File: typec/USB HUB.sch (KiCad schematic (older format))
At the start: 36 parts, among them U7 USB_HUB, Y1 24 MHz

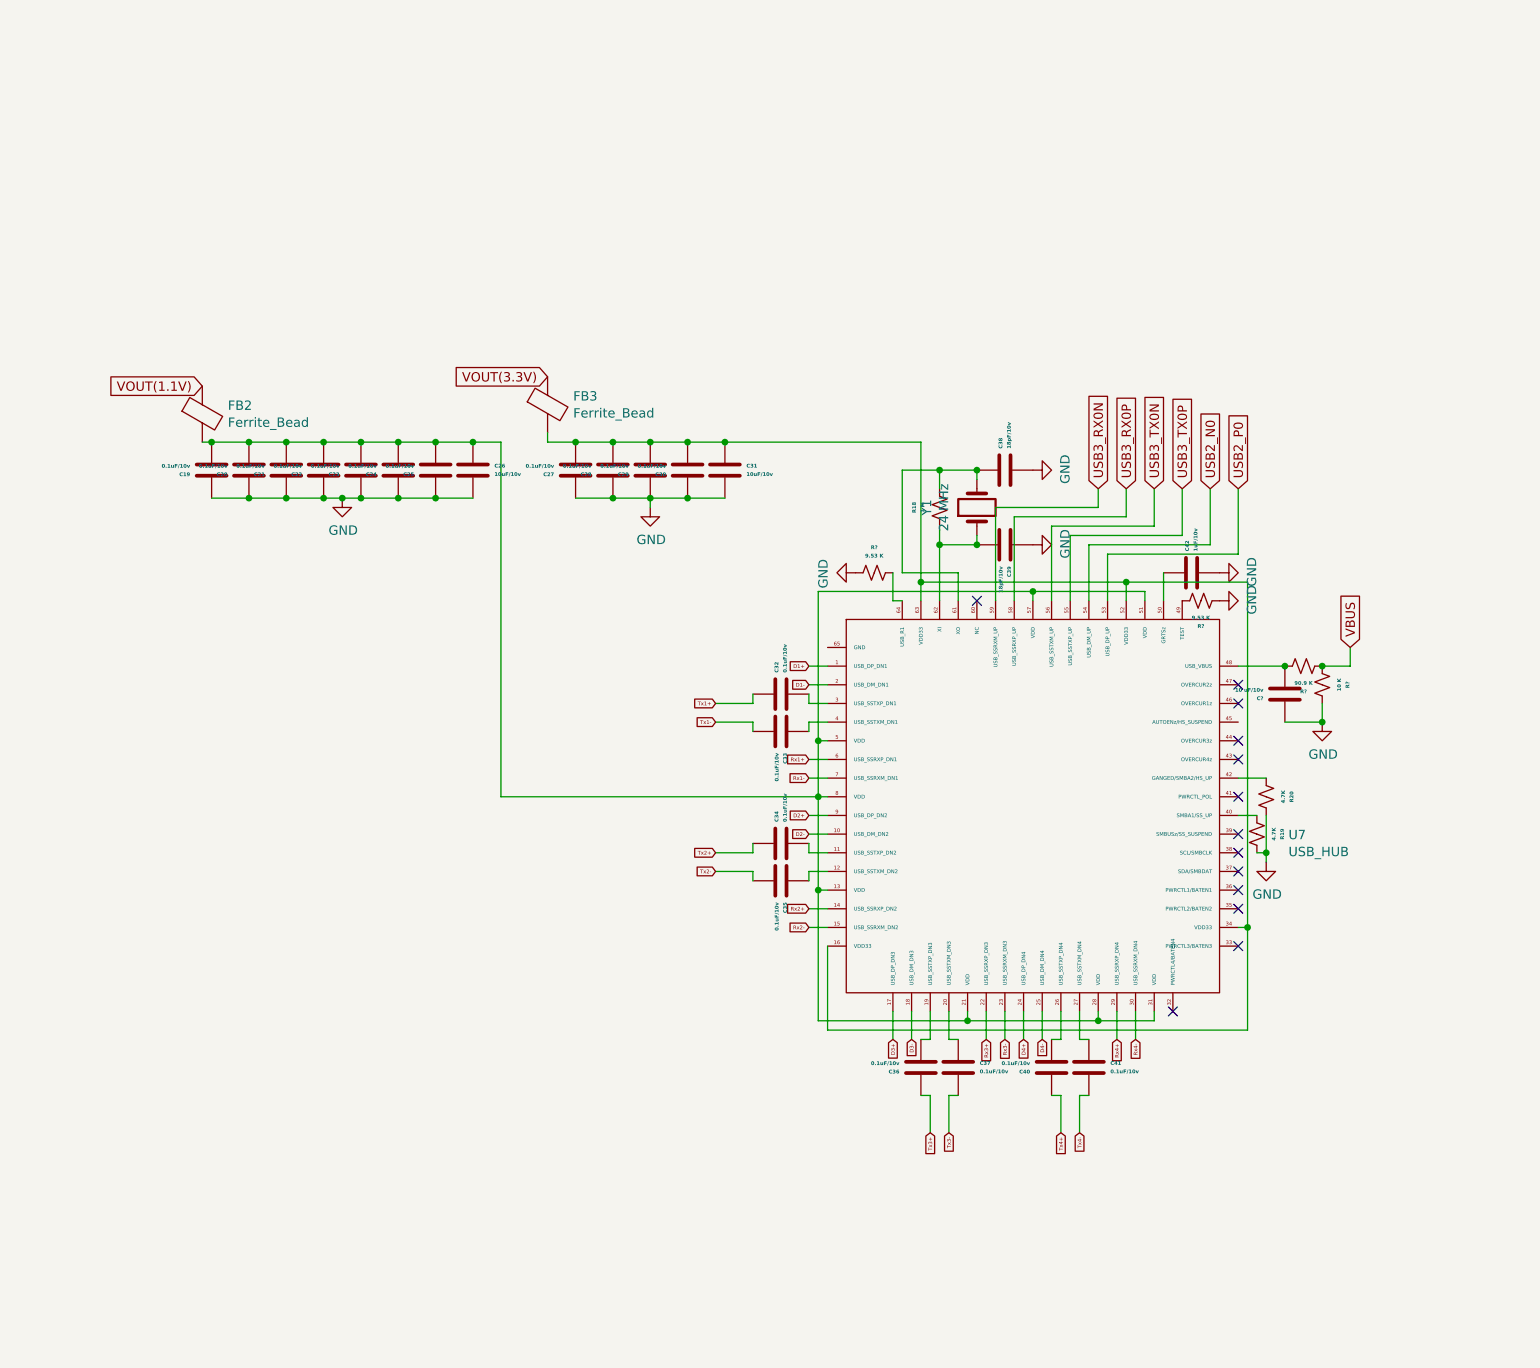
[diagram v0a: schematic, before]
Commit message: updated
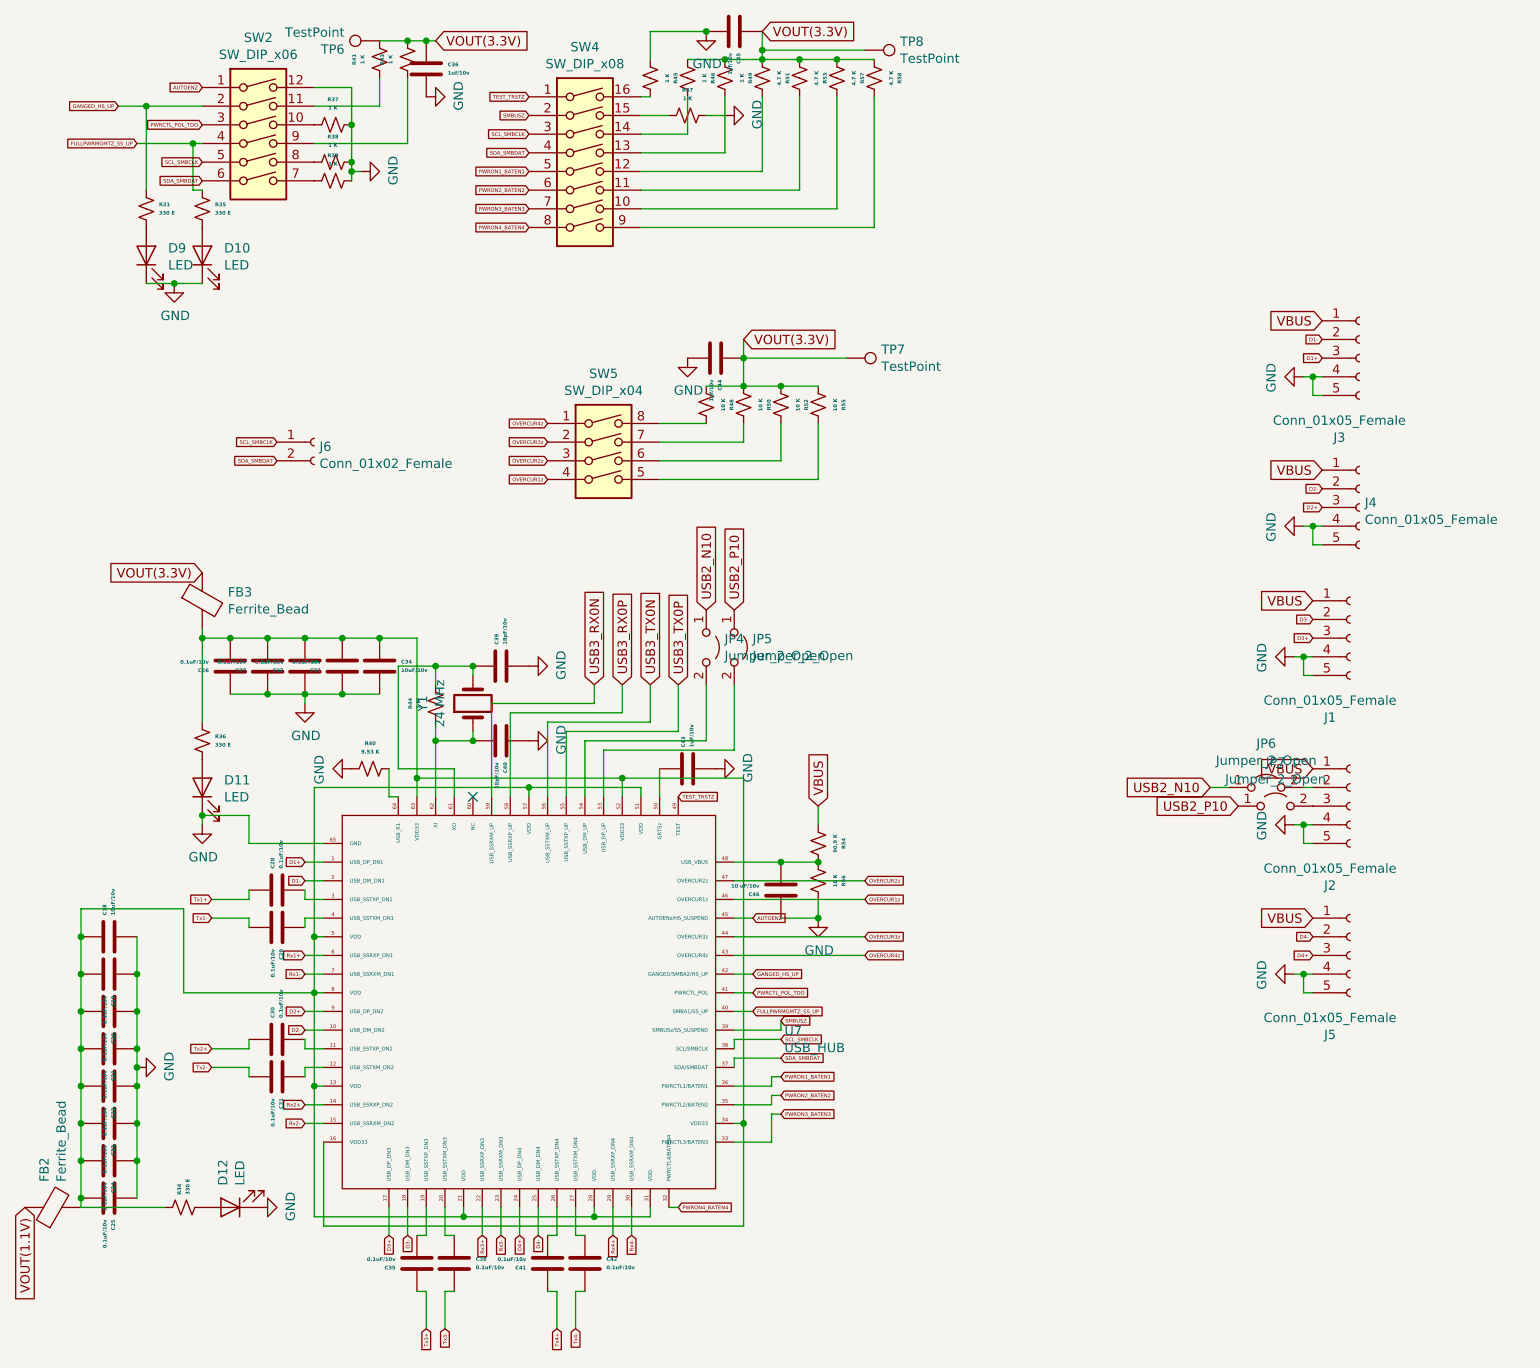
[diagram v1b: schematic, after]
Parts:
- removed R19, R20: 4.7K, Resistor_SMD:R_0402_1005Metric, symbol Device:R_Small_US
- removed R?: 9.53 K, Resistor_SMD:R_0402_1005Metric, symbol Device:R_Small_US
- added C36, C44, C45: 1uf/10v, Capacitor_SMD:C_0603_1608Metric, symbol Device:C
- added D10, D11, D12, D9: LED, LED_SMD:LED_0402_1005Metric, symbol Device:LED
- added J1, J2, J3, J4, J5: Conn_01x05_Female, Connector_JST:JST_GH_SM05B-GHS-TB_1x05-1MP_P1.25mm_Horizontal, symbol Connector:Conn_01x05_Female
- added J6: Conn_01x02_Female, Connector_PinHeader_1.00mm:PinHeader_1x02_P1.00mm_Vertical, symbol Connector:Conn_01x02_Female
- added JP4, JP5, JP6, JP7: Jumper_2_Open, Connector_PinHeader_1.00mm:PinHeader_1x02_P1.00mm_Vertical, symbol Jumper:Jumper_2_Open
- added R31, R34, R35, R36: 330 E, Resistor_SMD:R_0402_1005Metric, symbol Device:R_Small_US
- added R37, R38, R39, R41, R43, R45, R46, R47, R49: 1 K, Resistor_SMD:R_0402_1005Metric, symbol Device:R_Small_US
- added R48, R50, R52, R55: 10 K, Resistor_SMD:R_0402_1005Metric, symbol Device:R_Small_US
- added R51, R53, R57, R58: 4.7 K, Resistor_SMD:R_0402_1005Metric, symbol Device:R_Small_US
- added SW2: SW_DIP_x06, Button_Switch_THT:SW_DIP_SPSTx06_Slide_6.7x16.8mm_W7.62mm_P2.54mm_LowProfile, symbol Switch:SW_DIP_x06
- added SW4: SW_DIP_x08, Button_Switch_THT:SW_DIP_SPSTx08_Slide_6.7x21.88mm_W7.62mm_P2.54mm_LowProfile, symbol Switch:SW_DIP_x08
- added SW5: SW_DIP_x04, Button_Switch_THT:SW_DIP_SPSTx04_Slide_6.7x11.72mm_W7.62mm_P2.54mm_LowProfile, symbol Switch:SW_DIP_x04
- added TP6, TP7, TP8: TestPoint, TestPoint:TestPoint_THTPad_2.0x2.0mm_Drill1.0mm, symbol Connector:TestPoint
- C18: renamed from C26; footprint Capacitor_SMD:C_1206_3216Metric -> Capacitor_SMD:C_0603_1608Metric
- C19: renamed from C25; footprint Capacitor_SMD:C_1206_3216Metric -> Capacitor_SMD:C_0402_1005Metric
- C20: renamed from C24; footprint Capacitor_SMD:C_1206_3216Metric -> Capacitor_SMD:C_0402_1005Metric
- C21: renamed from C23; footprint Capacitor_SMD:C_1206_3216Metric -> Capacitor_SMD:C_0402_1005Metric
- C22: footprint Capacitor_SMD:C_1206_3216Metric -> Capacitor_SMD:C_0402_1005Metric
- C23: renamed from C21; footprint Capacitor_SMD:C_1206_3216Metric -> Capacitor_SMD:C_0402_1005Metric
- C24: renamed from C20; footprint Capacitor_SMD:C_1206_3216Metric -> Capacitor_SMD:C_0402_1005Metric
- C25: renamed from C19; footprint Capacitor_SMD:C_1206_3216Metric -> Capacitor_SMD:C_0402_1005Metric
- C26: renamed from C27; footprint Capacitor_SMD:C_1206_3216Metric -> Capacitor_SMD:C_0603_1608Metric
- C27: renamed from C28; footprint Capacitor_SMD:C_1206_3216Metric -> Capacitor_SMD:C_0603_1608Metric
- C28: renamed from C32; footprint Capacitor_SMD:C_0201_0603Metric -> Capacitor_SMD:C_0402_1005Metric
- C29: renamed from C33; footprint Capacitor_SMD:C_0201_0603Metric -> Capacitor_SMD:C_0402_1005Metric
- C30: renamed from C34; footprint Capacitor_SMD:C_0201_0603Metric -> Capacitor_SMD:C_0402_1005Metric
- C31: renamed from C35; footprint Capacitor_SMD:C_0201_0603Metric -> Capacitor_SMD:C_0402_1005Metric
- C32: renamed from C29; footprint Capacitor_SMD:C_1206_3216Metric -> Capacitor_SMD:C_0603_1608Metric
- C33: renamed from C30; footprint Capacitor_SMD:C_1206_3216Metric -> Capacitor_SMD:C_0603_1608Metric
- C34: renamed from C31; footprint Capacitor_SMD:C_1206_3216Metric -> Capacitor_SMD:C_0603_1608Metric
- C35: renamed from C36; footprint Capacitor_SMD:C_0201_0603Metric -> Capacitor_SMD:C_0402_1005Metric
- C38: renamed from C37; footprint Capacitor_SMD:C_0201_0603Metric -> Capacitor_SMD:C_0402_1005Metric
- C39: renamed from C38; footprint Capacitor_SMD:C_0603_1608Metric -> Capacitor_SMD:C_0201_0603Metric
- C40: renamed from C39; footprint Capacitor_SMD:C_0603_1608Metric -> Capacitor_SMD:C_0201_0603Metric
- C41: renamed from C40; footprint Capacitor_SMD:C_0201_0603Metric -> Capacitor_SMD:C_0402_1005Metric
- C42: renamed from C41; footprint Capacitor_SMD:C_0201_0603Metric -> Capacitor_SMD:C_0402_1005Metric
- C43: renamed from C42; footprint Capacitor_SMD:C_0805_2012Metric -> Capacitor_SMD:C_0603_1608Metric
- C46: renamed from C?; footprint Capacitor_SMD:C_0805_2012Metric -> Capacitor_SMD:C_0603_1608Metric
- R44: renamed from R18; footprint Resistor_SMD:R_0805_2012Metric -> Resistor_SMD:R_0402_1005Metric
- R54: renamed from R?; footprint Resistor_SMD:R_0805_2012Metric -> Resistor_SMD:R_0402_1005Metric
- gave numbers to parts that had none: 2
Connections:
- net D1+: now also J3.3 (Pin_3)
- net D1-: now also J3.2 (Pin_2)
- net D2+: now also J4.3 (Pin_3)
- net D2-: now also J4.2 (Pin_2)
- net D3+: now also J1.3 (Pin_3)
- net D3-: now also J1.2 (Pin_2)
- net D4+: now also J5.3 (Pin_3)
- net D4-: now also J5.2 (Pin_2)
- net GND: now also U7.65 (GND), C36.2, C44.2, C45.2, D10.1 (K), D11.1 (K), D12.1 (K), D9.1 (K), J1.4 (Pin_4), J1.5 (Pin_5), J2.4 (Pin_4), J2.5 (Pin_5), J3.4 (Pin_4), J3.5 (Pin_5), J4.4 (Pin_4), J4.5 (Pin_5), J5.4 (Pin_4), J5.5 (Pin_5), R37.1, R38.1, R39.1, R45.2, R47.1, SW2.12
- net VBUS: now also J1.1 (Pin_1), J2.1 (Pin_1), J3.1 (Pin_1), J4.1 (Pin_1), J5.1 (Pin_1); no longer R56.2
- net VOUT(3.3V): now also C36.1, C44.1, C45.1, R41.1, R43.1, R46.2, R48.2, R49.2, R50.2, R51.2, R52.2, R53.2, R55.2, R57.2, R58.2, TP6.1, TP7.1, TP8.1
- net at C46.2, R54.1, U7.48 (USB_VBUS): now also R56.2
- net at C18.1, C19.2, C20.2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: now also R34.1
- net at C26.2, C27.2, C32.2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: now also R36.1
- net PWRON4_BATEN4: now reaches U7.32 (PWRCTL4/BATEN4)
- net PWRON4_BATEN4: now also SW4.8
- net PWRON3_BATEN3: now reaches U7.33 (PWRCTL3/BATEN3)
- net PWRON3_BATEN3: now also SW4.7
- net PWRON2_BATEN2: now reaches U7.35 (PWRCTL2/BATEN2)
- net PWRON2_BATEN2: now also SW4.6
- net PWRON1_BATEN1: now reaches U7.36 (PWRCTL1/BATEN1)
- net PWRON1_BATEN1: now also SW4.5
- net SDA_SMBDAT: now reaches U7.37 (SDA/SMBDAT)
- net SDA_SMBDAT: now also J6.2 (Pin_2), SW2.6, SW4.4
- net SCL_SMBCLK: now reaches U7.38 (SCL/SMBCLK)
- net SCL_SMBCLK: now also J6.1 (Pin_1), SW2.5, SW4.3
- net SMBUSZ: now reaches U7.39 (SMBUSz/SS_SUSPEND)
- net SMBUSZ: now also SW4.2
- net FULLPWRMGMTZ_SS_UP: now reaches U7.40 (SMBA1/SS_UP)
- net FULLPWRMGMTZ_SS_UP: now also R35.1, SW2.4
- net PWRCTL_POL_TDO: now reaches U7.41 (PWRCTL_POL)
- net PWRCTL_POL_TDO: now also SW2.3
- net GANGED_HS_UP: now reaches U7.42 (GANGED/SMBA2/HS_UP)
- net GANGED_HS_UP: now also R31.1, SW2.2
- net OVERCUR4z: now reaches U7.43 (OVERCUR4z)
- net OVERCUR4z: now also SW5.1
- net OVERCUR3z: now reaches U7.44 (OVERCUR3z)
- net OVERCUR3z: now also SW5.2
- net AUTOENZ: now reaches U7.45 (AUTOENz/HS_SUSPEND)
- net AUTOENZ: now also SW2.1
- net OVERCUR1z: now reaches U7.46 (OVERCUR1z)
- net OVERCUR1z: now also SW5.4
- net OVERCUR2z: now reaches U7.47 (OVERCUR2z)
- net OVERCUR2z: now also SW5.3
- net TEST_TRSTZ: now reaches U7.49 (TEST)
- net TEST_TRSTZ: now also SW4.1
- net USB2_N0: no longer names the net of U7.54 (USB_DM_UP)
- net USB2_N0: now also JP4.2 (B)
- net USB2_P0: no longer names the net of U7.53 (USB_DP_UP)
- net USB2_P0: now also JP5.2 (B)
- new net: R57.1, SW4.10
- new net: R53.1, SW4.11
- new net: R51.1, SW4.12
- new net: R49.1, SW4.13
- new net: R46.1, SW4.14
- new net: R47.2, SW4.15
- new net: R45.1, SW4.16
- new net: R58.1, SW4.9
- new net: J2.3 (Pin_3), JP7.2 (B)
- new net: J2.2 (Pin_2), JP6.2 (B)
- new net: R38.2, SW2.8
- new net: R39.2, SW2.7
- new net: R41.2, SW2.11
- new net: R37.2, SW2.10
- new net: R43.2, SW2.9
- new net: D9.2 (A), R31.2
- new net: D10.2 (A), R35.2
- new net: D11.2 (A), R36.2
- new net: D12.2 (A), R34.2
- new net: R52.1, SW5.6
- new net: R50.1, SW5.7
- new net: R48.1, SW5.8
- new net: R55.1, SW5.5
- new net USB2_N10: JP4.1 (A), JP6.1 (A)
- new net USB2_P10: JP5.1 (A), JP7.1 (A)
- no-connect marks 13 -> 1
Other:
- moved on the sheet: C18, C19, C20, C21, C22, C23, C24, C25, C26, C27, C28, C29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
